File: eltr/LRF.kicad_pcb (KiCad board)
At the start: 2 copper layers, 5 parts, among them P1 CONN_01X04, Q1 PN2222A

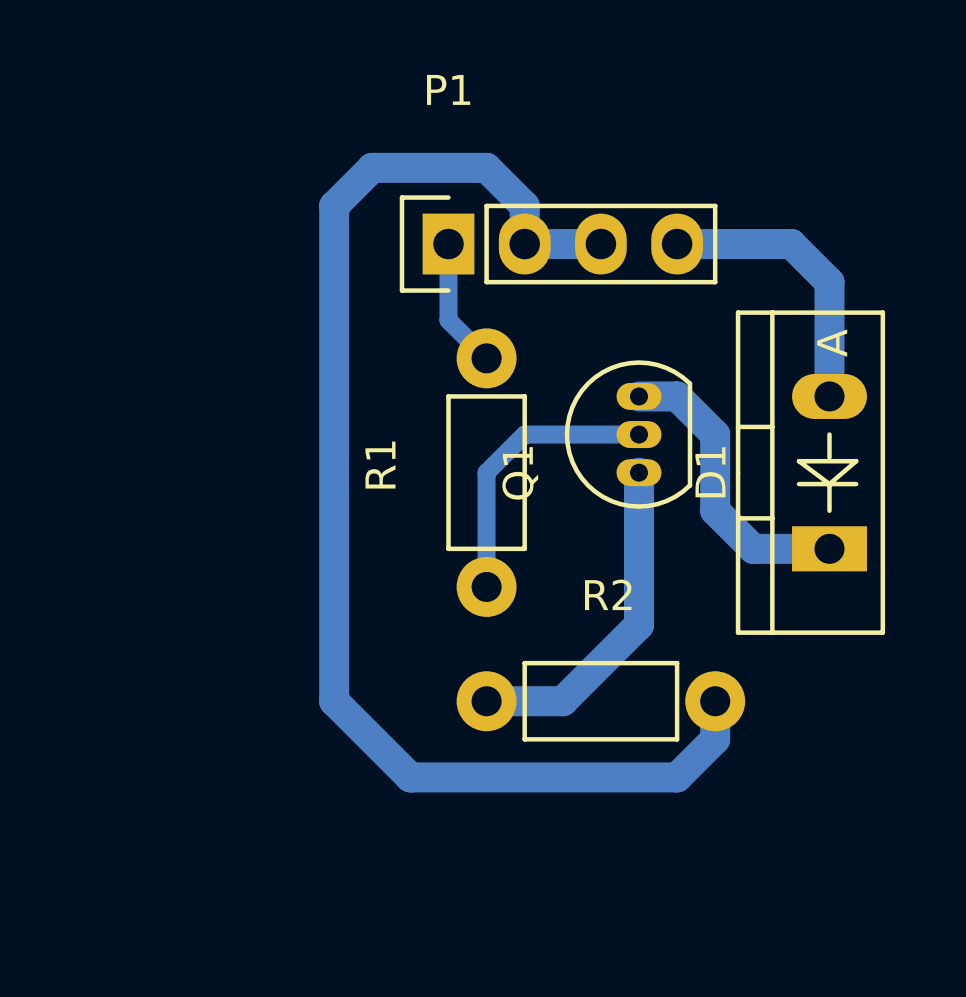
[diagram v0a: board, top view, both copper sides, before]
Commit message: Cleaning up
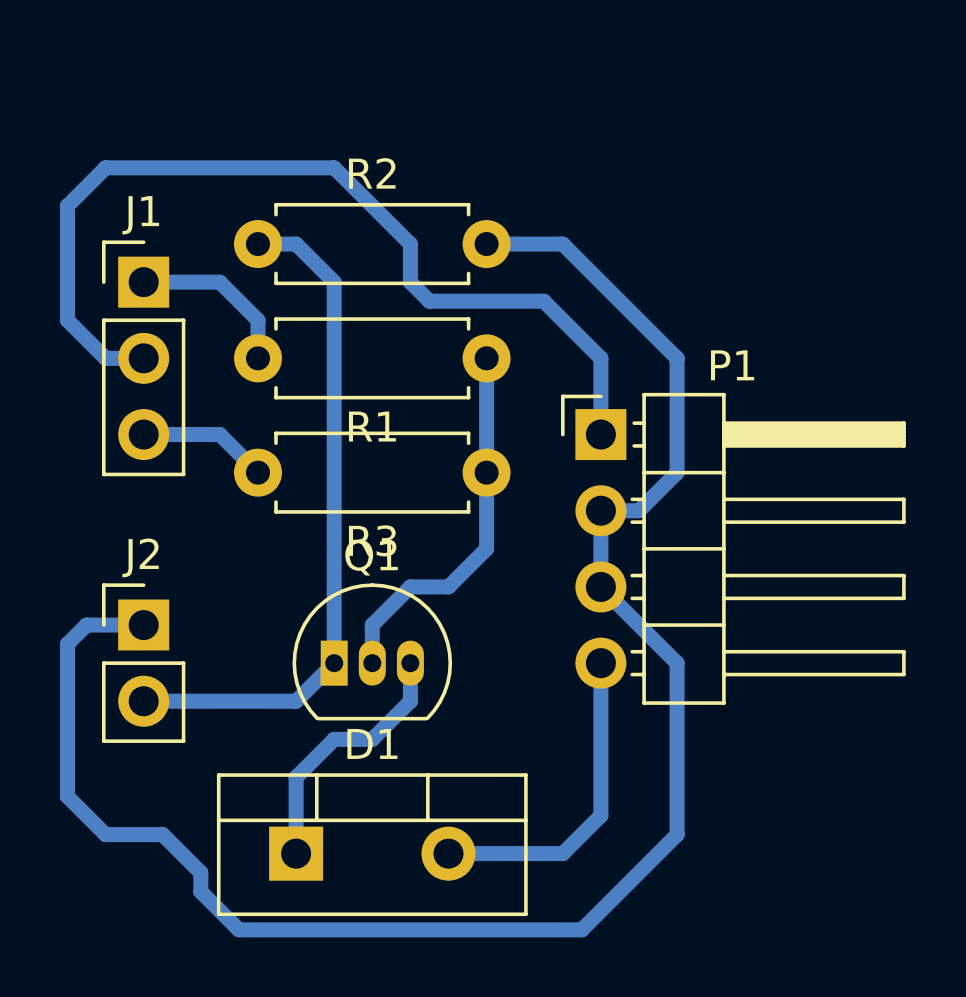
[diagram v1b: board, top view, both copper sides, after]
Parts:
- added J1: CONN_01X03_MALE, Pin_Headers:Pin_Header_Straight_1x03_Pitch2.54mm, F.Cu at (147.3, 100.3)
- added J2: CONN_01X02_MALE, Pin_Headers:Pin_Header_Straight_1x02_Pitch2.54mm, F.Cu at (147.3, 111.8)
- added R3: 1K, Resistors_THT:R_Axial_DIN0207_L6.3mm_D2.5mm_P7.62mm_Horizontal, F.Cu at (158.8, 106.7)
- D1: footprint Diodes_ThroughHole:Diode_TO-220_Vertical -> TO_SOT_Packages_THT:TO-220-2_Vertical
- P1: footprint Socket_Strips:Socket_Strip_Straight_1x04 -> Pin_Headers:Pin_Header_Angled_1x04_Pitch2.54mm
- R1, R2: footprint Resistors_ThroughHole:Resistor_Horizontal_RM7mm -> Resistors_THT:R_Axial_DIN0207_L6.3mm_D2.5mm_P7.62mm_Horizontal
- moved D1 20.5 mm to (152.4, 119.4), turned to 0 degrees
- moved R2 17.0 mm to (151.1, 99.1)
- moved Q1 12.0 mm to (153.7, 113.0), turned to 0 degrees
- moved P1 8.13 mm to (162.6, 105.4)
- moved R1 7.62 mm to (158.8, 102.9), turned to 180 degrees
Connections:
- R1 pad 2: GPIO -> Net-(J1-Pad1)
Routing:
- net GPIO: track 4.34 -> 31.1 mm
- net GND: track 43.3 -> 58.4 mm
- net Net-(J2-Pad2): track 11.2 -> 22.6 mm
- net Net-(J1-Pad1): track 0.00 -> 5.61 mm
- net Net-(J1-Pad3): track 0.00 -> 4.34 mm
- net Net-(Q1-Pad2): track 9.42 -> 12.5 mm
- net Net-(D1-Pad1): track 9.94 -> 8.67 mm
- net +5V: track 9.42 -> 10.7 mm
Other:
- net class Default: clearance 0.25 -> 0.2; trace_width 1 -> 0.5
- rule pad_to_mask_clearance: 0.2 -> 0
- rule trace_clearance: 0.25 -> 0.2
- rule trace_min: 0.5 -> 0.2
